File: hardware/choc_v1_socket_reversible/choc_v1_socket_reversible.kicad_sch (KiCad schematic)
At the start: 76 parts, among them J1 Conn_01x12_MountingPin, J2 Conn_01x12_MountingPin, SW00 SW_Push, SW01 SW_Push, SW02 SW_Push, SW03 SW_Push, SW04 SW_Push, SW05 SW_Push, SW10 SW_Push, SW11 SW_Push, SW12 SW_Push, SW13 SW_Push, SW14 SW_Push, SW15 SW_Push, SW20 SW_Push, SW21 SW_Push, SW22 SW_Push, SW23 SW_Push, SW24 SW_Push, SW25 SW_Push, SW30 SW_Push, SW31 SW_Push, SW32 SW_Push, SW33 SW_Push, SW34 SW_Push, SW35 SW_Push, SW36 SW_Push, SW37 SW_Push, U1 CH582

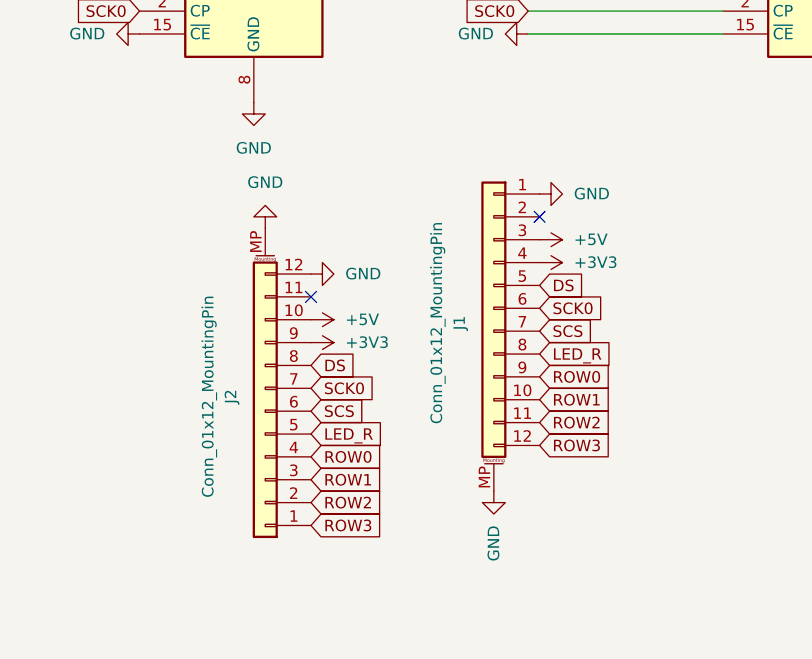
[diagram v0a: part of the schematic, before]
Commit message: Generated gerber
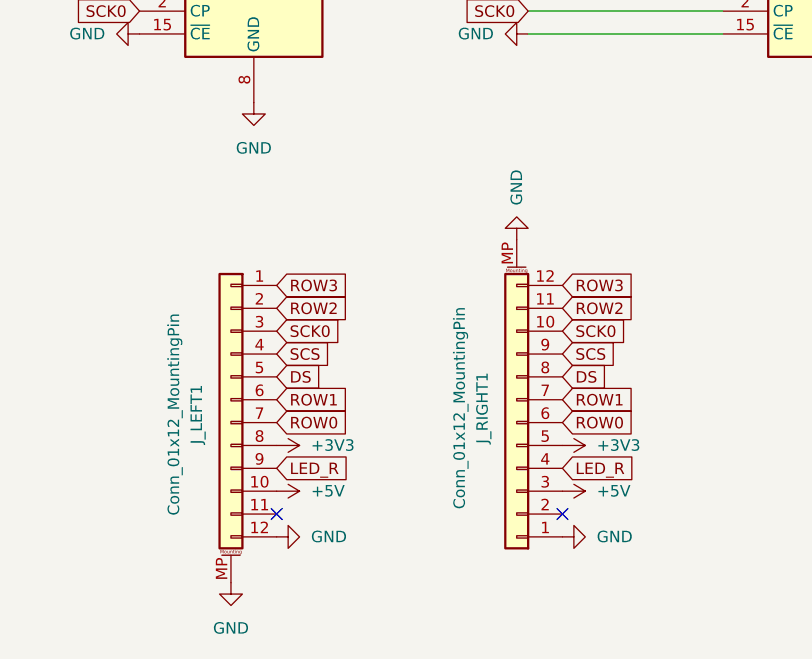
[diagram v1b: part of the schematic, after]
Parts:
- renumbered J2 to J_LEFT1, J1 to J_RIGHT1
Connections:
- net +3V3: now also J_LEFT1.8 (Pin_8), J_RIGHT1.5 (Pin_5); no longer J_LEFT1.9 (Pin_9), J_RIGHT1.4 (Pin_4)
- net DS: now also J_LEFT1.5 (Pin_5), J_RIGHT1.8 (Pin_8); no longer J_LEFT1.8 (Pin_8), J_RIGHT1.5 (Pin_5)
- net LED_R: now also J_LEFT1.9 (Pin_9), J_RIGHT1.4 (Pin_4); no longer J_LEFT1.5 (Pin_5), J_RIGHT1.8 (Pin_8)
- net ROW0: now also J_LEFT1.7 (Pin_7), J_RIGHT1.6 (Pin_6); no longer J_LEFT1.4 (Pin_4), J_RIGHT1.9 (Pin_9)
- net ROW1: now also J_LEFT1.6 (Pin_6), J_RIGHT1.7 (Pin_7); no longer J_LEFT1.3 (Pin_3), J_RIGHT1.10 (Pin_10)
- net SCK0: now also J_LEFT1.3 (Pin_3), J_RIGHT1.10 (Pin_10); no longer J_LEFT1.7 (Pin_7), J_RIGHT1.6 (Pin_6)
- net SCS: now also J_LEFT1.4 (Pin_4), J_RIGHT1.9 (Pin_9); no longer J_LEFT1.6 (Pin_6), J_RIGHT1.7 (Pin_7)
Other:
- moved on the sheet: J_LEFT1, J_RIGHT1
